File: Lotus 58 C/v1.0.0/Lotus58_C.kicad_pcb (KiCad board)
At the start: 2 copper layers, 139.1 x 107.7 mm, 137 parts, among them J1 USB_C_Receptacle_USB2.0, J2 Conn_01x02, J3 USB_C_Receptacle_USB2.0, P1 OLED, Q1 AO3401A, SW1 Kailh hotswap MX socket, SW10 Kailh hotswap MX socket, SW11 Kailh hotswap MX socket, SW12 Kailh hotswap MX socket, SW13 Kailh hotswap MX socket, SW14 Kailh hotswap MX socket, SW15 Kailh hotswap MX socket, SW16 Kailh hotswap MX socket, SW17 Kailh hotswap MX socket, SW18 Kailh hotswap MX socket, SW19 Kailh hotswap MX socket, SW2 Kailh hotswap MX socket, SW20 Kailh hotswap MX socket, SW21 Kailh hotswap MX socket, SW22 Kailh hotswap MX socket, SW23 Kailh hotswap MX socket, SW24 Kailh hotswap MX socket, SW25 Kailh hotswap MX socket, SW26 Kailh hotswap MX socket, SW27 Kailh hotswap MX socket, SW28 Kailh hotswap MX socket, SW29 Kailh hotswap MX socket, SW3 Kailh hotswap MX socket, SW30 Rotary_Encoder_Switch, SW31 Rotary_Encoder_Switch, SW4 Kailh hotswap MX socket, SW5 Kailh hotswap MX socket, SW6 Kailh hotswap MX socket, SW7 Kailh hotswap MX socket, SW8 Kailh hotswap MX socket, SW9 Kailh hotswap MX socket, U1 ProMicro, U2 SRV05-4

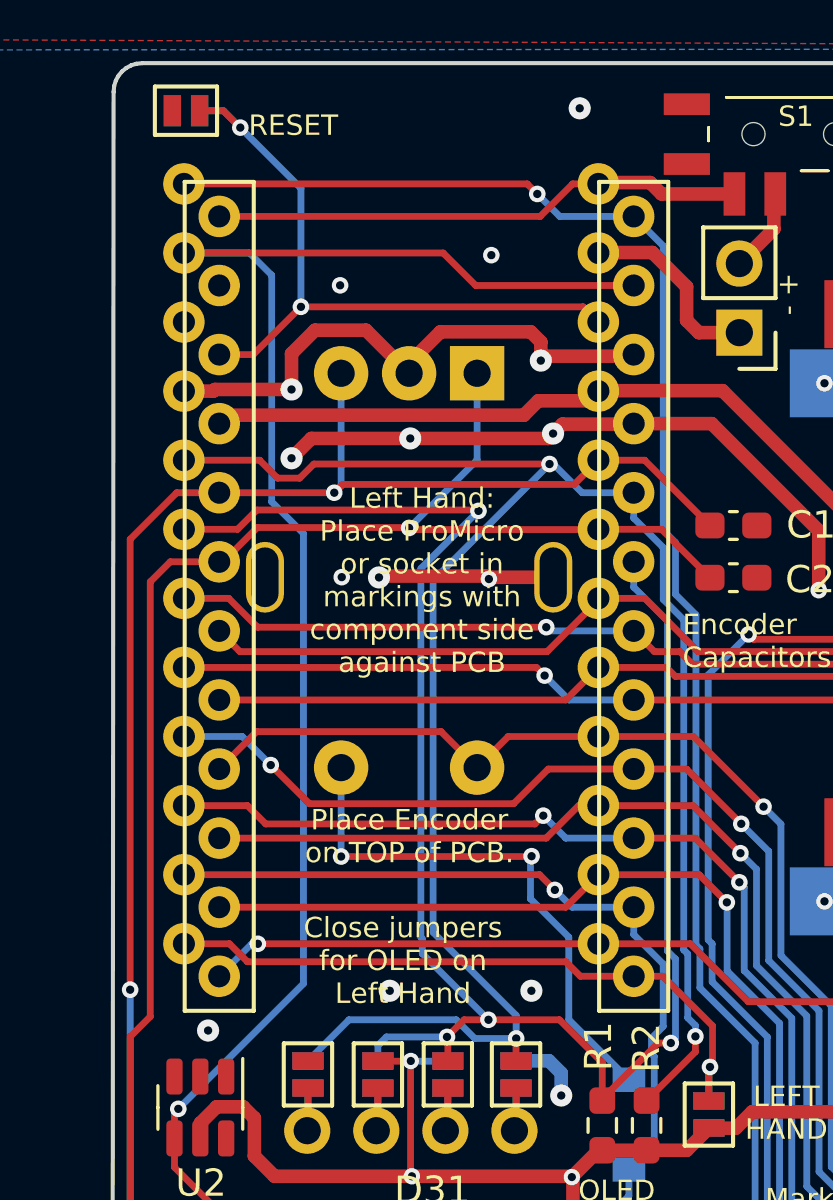
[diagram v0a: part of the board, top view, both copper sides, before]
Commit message: General cleanup and rename
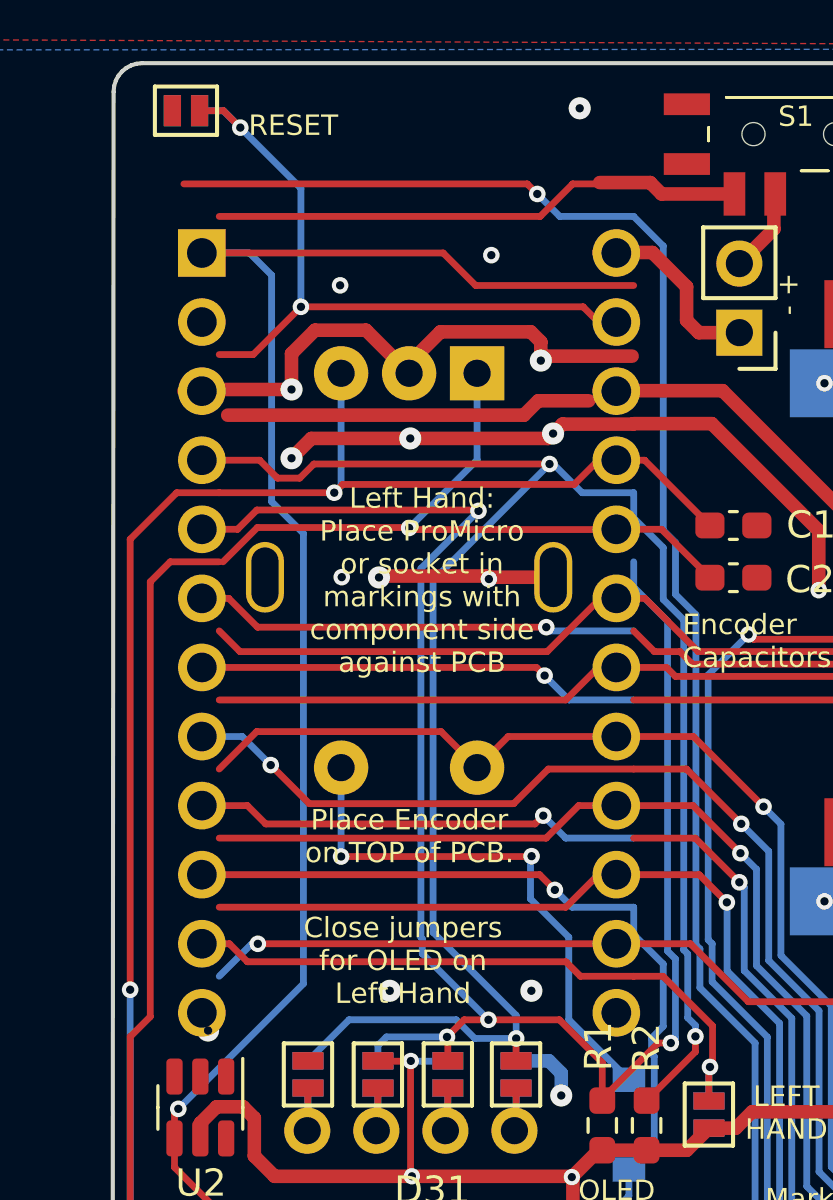
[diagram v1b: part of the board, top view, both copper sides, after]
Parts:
- U1: footprint Keyboard Library:ProMicro_Reversible -> Keyboard Controllers:ProMicro-FrontSide
- moved U1 1.82 mm to (91.6, 56.6), turned to -90 degrees
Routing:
- net GND: track 191.8 -> 168.1 mm, vias 99 -> 94
- net VCC: track 869.5 -> 893.2 mm, vias 47 -> 51
- net row3: track 176.0 -> 158.7 mm, vias 9 -> 8
- net row2: track 159.5 -> 176.8 mm, vias 9 -> 10
- net row1: track 144.1 -> 127.1 mm, vias 7 -> 6
- net SCL: track 65.7 -> 82.7 mm, vias 4 -> 5
- net Hand: vias 1 -> 2
